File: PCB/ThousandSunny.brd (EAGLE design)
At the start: 101 x 87.7 mm, 26 parts, among them IC1 LM317LZ

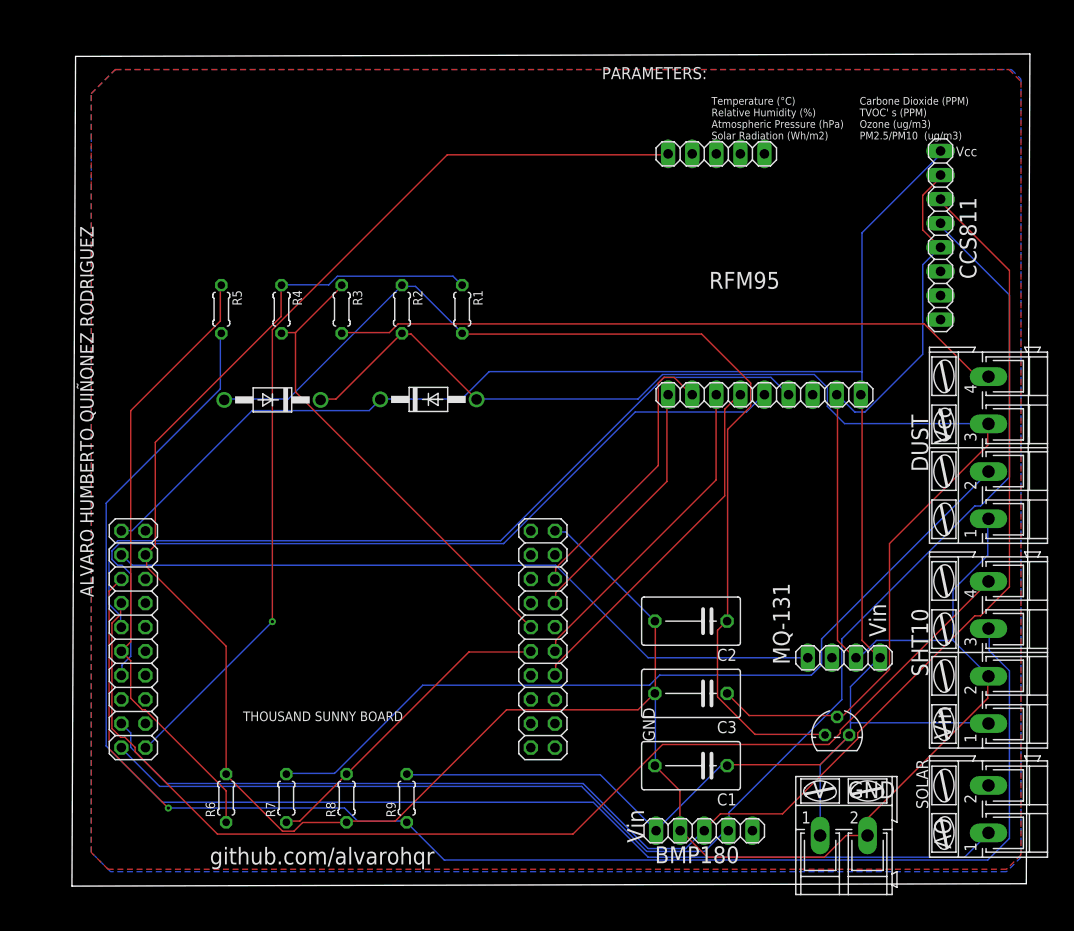
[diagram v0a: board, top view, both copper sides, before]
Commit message: Board Bill of Materials
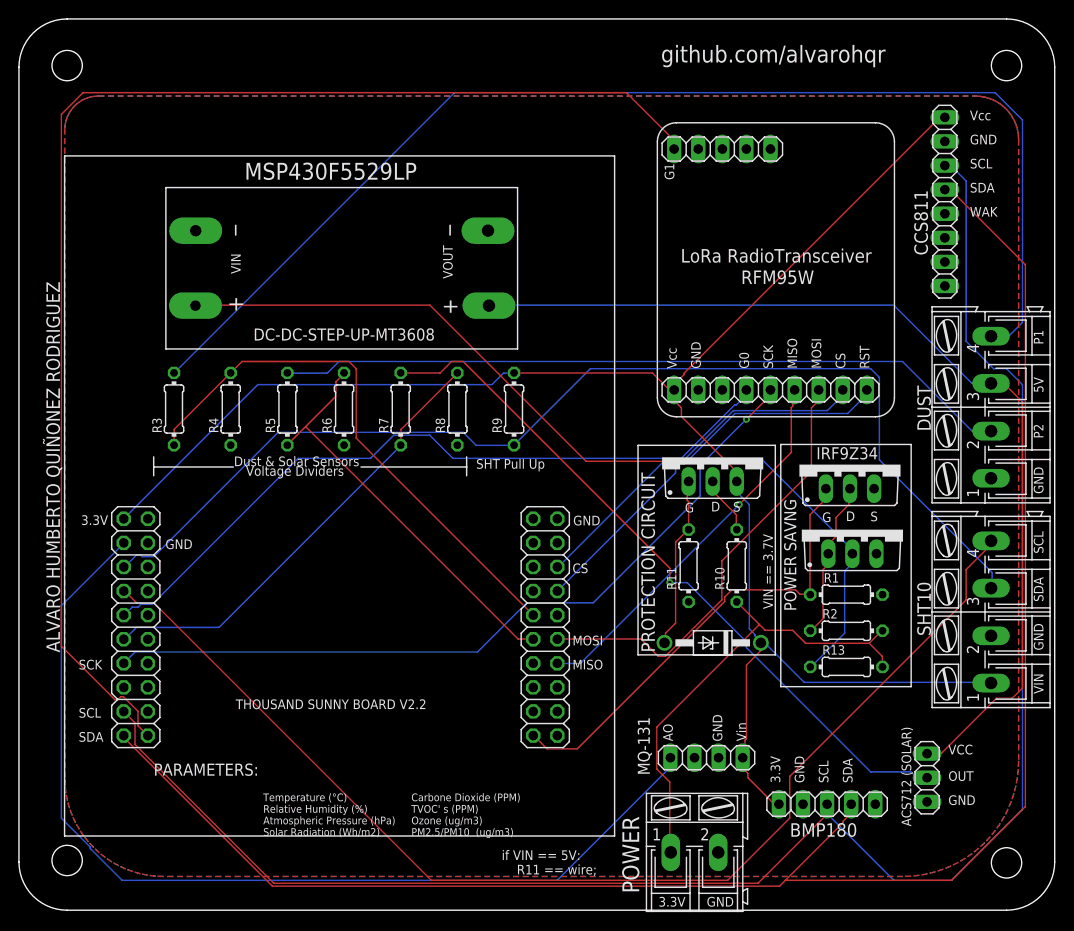
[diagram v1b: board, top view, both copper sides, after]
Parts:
- removed C1: 0.1uF, rcl:C075-052X106
- removed C2: 10 uF, rcl:C075-052X106
- removed C3: 1 uF, rcl:C075-052X106
- removed D1: 1N4002, diode:DO41-10
- removed IC1: LM317LZ, linear:TO92
- removed X3, X4: (no value), con-ptr500:AK300/2
- added IRF9Z34, IRF9Z34_#2: IRF540, transistor-power:TO220BV
- added JP8: (no value), pinhead:1X03
- added POWER: (no value), con-ptr500:AK300/2
- added Q1: IRF9Z34N, transistor-power:TO220BV
- added R10: 330 Ω, resistor:0204/7
- added R11: 10 kΩ, resistor:0204/7
- added R13: 100 Ω, resistor:0204/7
- added U$1: DC-DC-STEP-UP-MT3608, dc-dc-boost-2a-microusb-mt3608:DC-DC-STEP-UP-MT3608
- D2: value 1N4002 -> 1N4728; device diode:DO41-10 -> diode:DO41Z10
- R1: value 720 Ω -> 10 kΩ; device rcl:0204/5 -> resistor:0204/7
- R2: value 240 Ω -> 100 Ω; device rcl:0204/5 -> resistor:0204/7
- R3, R5, R7: value 1 kΩ -> 100 Ω; device rcl:0204/5 -> resistor:0204/7
- R4, R6, R8: value 1.8 kΩ -> 220 Ω; device rcl:0204/5 -> resistor:0204/7
- R9: value 5.1 kΩ -> 10 kΩ; device rcl:0204/5 -> resistor:0204/7
- moved R2 57.8 mm to (82.2, 26.9), turned to 0 degrees
- moved D2 53.0 mm to (68.1, 25.7)
- moved R1 50.5 mm to (82.2, 30.7), turned to 180 degrees
- moved R6 42.9 mm to (29.2, 50.3), turned to 90 degrees
- moved R7 42.8 mm to (35.2, 50.3)
- moved R8 42.7 mm to (41.2, 50.3)
- moved R9 42.6 mm to (47.1, 50.3)
- moved R3 20.6 mm to (11.3, 50.3), turned to 90 degrees
- moved JP7 17.9 mm to (67.4, 13.5)
- moved JP4 13.3 mm to (80.1, 8.64)
- moved R5 12.6 mm to (23.2, 50.3), turned to 90 degrees
- moved R4 11.8 mm to (17.2, 50.3), turned to 90 degrees
- moved X1 4.28 mm to (97.4, 28.9)
- moved X2 4.28 mm to (97.4, 50.5)
- moved JP3 3.57 mm to (92.6, 72.2)
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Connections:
- net N$15 renamed RAW_P1
- net P1.3 renamed DUST_P1
- net P1.6 renamed RFM95W_G0
- net P2.2 renamed RFM95W_CS
- net P3.0 renamed MOSI
- net P3.1 renamed MISO
- net P3.2 renamed SCK
- net P3.3 renamed SHT_CLOCK
- net P3.4 renamed SHT_DATA
- net P3.5 renamed G1
- net P4.1 renamed SDA
- net P4.2 renamed SCL
- net P6.5 renamed O3
- net P7.4 renamed RFM95_RST
- removed net N$17: R7.2, X2.2
- removed net N$18: R5.2, X3.1
- removed net N$2: C2.1, D2.A, IC1.1, R1.2, R2.1
- removed net P1.2: JP2.11, R7.1, R8.2
- removed net P6.6: JP1.11, R5.1, R6.2
- removed net VIN: C1.1, D1.C, IC1.3, JP1.1, JP3.1, JP4.1, JP6.9, JP7.4, R9.2, X1.1, X4.1
- removed net VO: C3.1, D1.A, D2.C, IC1.2, R2.2, X2.3
- new net ANODE: D2.A, Q1.G, R11.2
- new net BATTERY: POWER.1, R10.1, R13.2, R2.2
- new net D1->G2: IRF9Z34.D, IRF9Z34_#2.G, R2.1
- new net D2->VIN: IRF9Z34_#2.D, R13.1, U$1.IN+
- new net DRAIN_Q1: Q1.D, R10.2
- new net DUST_P2: JP2.11, R5.1, R6.2
- new net P8.2: IRF9Z34.G, JP2.19, R1.2
- new net RAW_P2: R5.2, X2.2
- new net RAW_SOLAR: JP8.2, R7.2
- new net SOLAR: JP1.11, R7.1, R8.2
- new net VIN->DUST: JP8.1, U$1.OUT+, X2.3
- new net VZ->3.3V: D2.C, JP1.1, JP3.1, JP4.1, JP6.9, JP7.4, Q1.S, R9.2, X1.1
- net GND: now also IRF9Z34.S, IRF9Z34_#2.S, JP8.3, POWER.2, R11.1, U$1.IN-, U$1.OUT-; no longer C1.2, C2.2, C3.2, X4.2
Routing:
- net GND: track 309.5 -> 0.00 mm
- net VIN: track 232.4 -> 0.00 mm
- net VZ->3.3V: track 0.00 -> 182.3 mm
- net N$18: track 147.5 -> 0.00 mm
- net VO: track 131.1 -> 0.00 mm
- net N$2: track 112.4 -> 0.00 mm
- net VIN->DUST: track 0.00 -> 103.6 mm
- net D2->VIN: track 0.00 -> 94.2 mm, vias 0 -> 1
- net N$17: track 88.9 -> 0.00 mm
- net RAW_P2: track 0.00 -> 77.7 mm
- net RAW_SOLAR: track 0.00 -> 75.4 mm, vias 0 -> 1
- net P6.6: track 65.8 -> 0.00 mm
- net RAW_P1: track 71.0 -> 128.2 mm
- net BATTERY: track 0.00 -> 50.0 mm
- net P8.2: track 0.00 -> 49.0 mm
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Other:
- board size 101 x 87.7 mm -> 109.2 x 94 mm
- board text added: "+"
- board text added: "3.3V"
- board text added: "5V"
- board text added: "ACS712 (SOLAR)"
- board text added: "CS"
- board text added: "D"
- board text added: "Dust & Solar Sensors"
- board text added: "G"
- board text added: "G0"
- board text added: "G1"
- board text added: "LoRa RadioTransceiver"
- board text added: "MISO"
- board text added: "MOSI"
- board text added: "MSP430F5529LP"
- board text added: "OUT"
- board text added: "P1"
- board text added: "P2"
- board text added: "POWER"
- board text added: "POWER SAVNG"
- board text added: "PROTECTION CIRCUIT"
- board text added: "RFM95W"
- board text added: "RST"
- board text added: "S"
- board text added: "SCK"
- board text added: "SCL"
- board text added: "SDA"
- board text added: "SHT Pull Up"
- board text added: "THOUSAND SUNNY BOARD V2"
- board text added: "THOUSAND SUNNY BOARD V2.2"
- board text added: "VCC"
- board text added: "VIN"
- board text added: "VIN == 3.7V"
- board text added: "VOUT"
- board text added: "Voltage Dividers"
- board text added: "WAK"
- board text added: "_"
- board text added: "if VIN == 5V: R11 == wire;"
- board text removed: "RFM95"
- board text removed: "SOLAR"
- board text removed: "THOUSAND SUNNY BOARD"
- board text removed: "V"
